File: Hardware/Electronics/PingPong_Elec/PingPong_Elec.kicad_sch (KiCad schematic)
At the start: 16 parts, among them M1 JGA25-371 12V, M2 JGA25-371 12V, M3 JGA25-371 12V, M4 MG996R, M5 MG996R, M6 MG996R, U1 DRV8871, U2 PCA9685PW, U5 DRV8871, U6 STM32F103RBTx LQFP64, U7 DRV8871

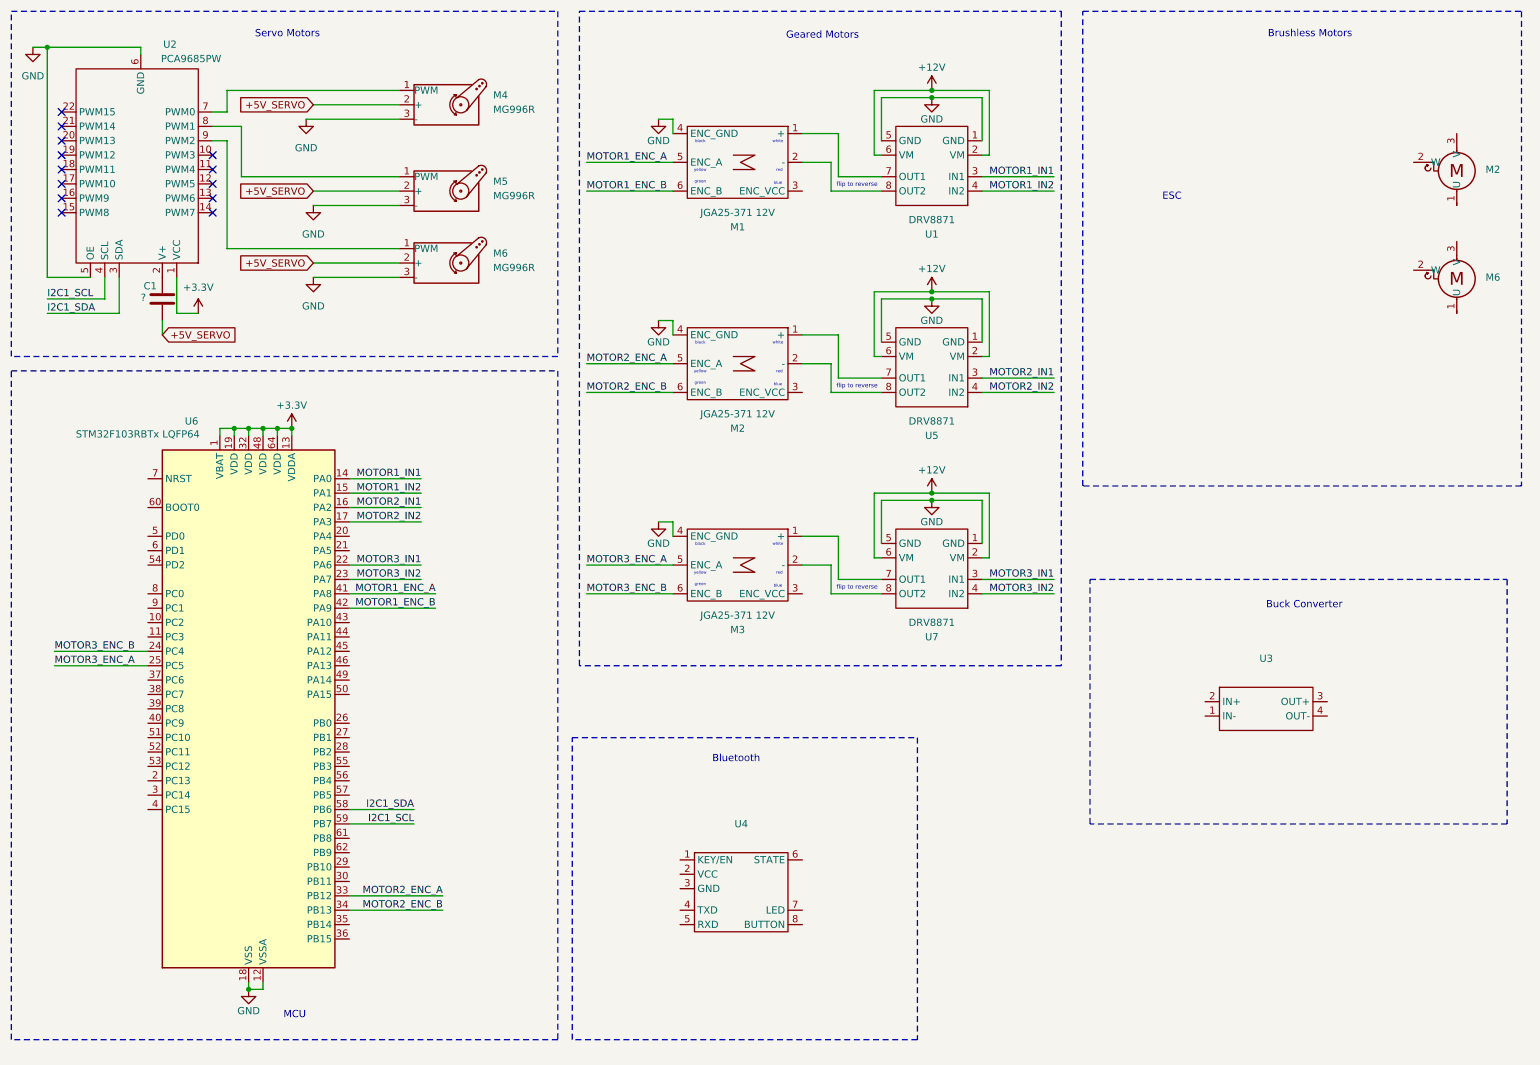
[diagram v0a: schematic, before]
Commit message: wired all schematic diagrams, adding bypass and decoupling caps
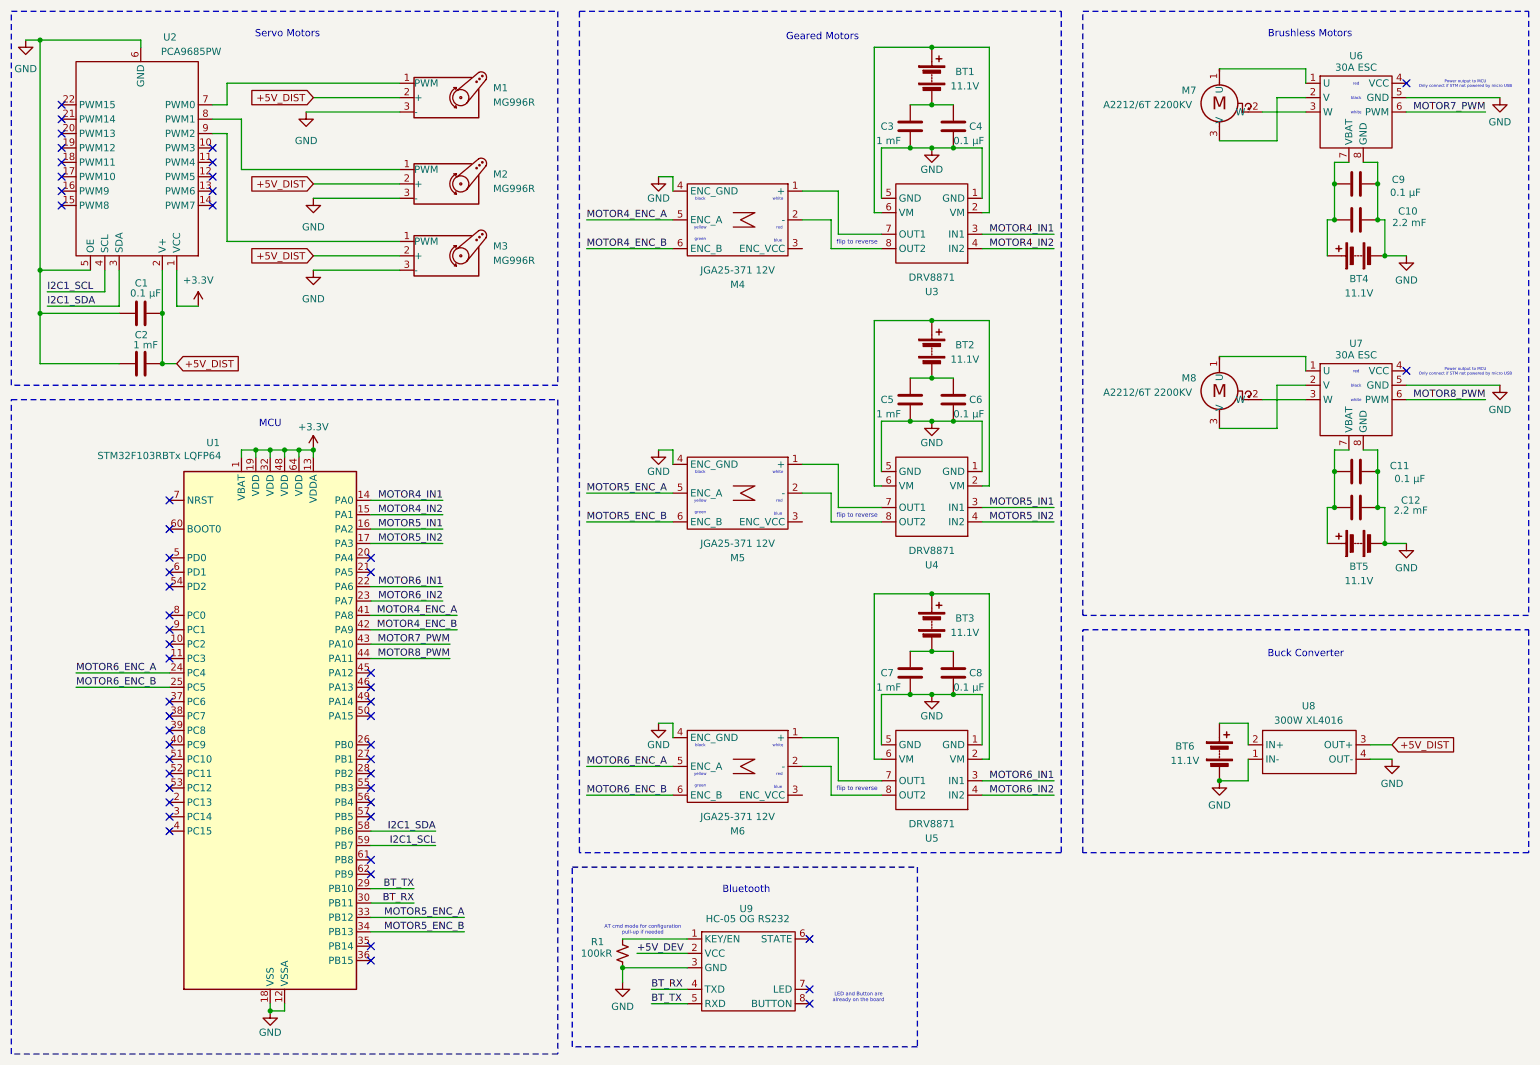
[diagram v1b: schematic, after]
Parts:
- removed M6: ~, symbol Motors:Motor_BLDC_3Phase
- added BT1, BT2, BT3, BT4, BT5, BT6: 11.1V, symbol Device:Battery
- added C1, C11, C4, C6, C8, C9: 0.1 µF, symbol Device:C
- added C10, C12: 2.2 mF, symbol Device:C
- added C3, C5, C7: 1 mF, symbol Device:C
- added M8: A2212/6T 2200KV, symbol Motors:Motor_BLDC_3Phase
- added R1: 100kR, symbol Device:R_Small_US
- added U6, U7: 30A ESC, symbol Motors:3Phase_ESC
- C2: renamed from C1; value ? -> 1 mF
- M7: renamed from M2; value ~ -> A2212/6T 2200KV
- U8: renamed from U3; value ~ -> 300W XL4016
- U9: renamed from U4; value ~ -> HC-05 OG RS232
- renumbered M4 to M1, M5 to M2, M6 to M3, M1 to M4, M2 to M5, M3 to M6, U6 to U1, U1 to U3, U5 to U4, U7 to U5
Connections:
- net +5V_SERVO is gone; now on net +5V_DIST: C2.2, M1.2 (+), M2.2 (+), M3.2 (+)
- net GND: now also C2.1, U8.1 (IN-), U8.4 (OUT-), U9.3 (GND), BT4.2 (-), BT5.2 (-), BT6.2 (-), C1.1, C10.2, C11.1, C12.2, C3.1, C4.1, C5.1, C6.1, C7.1, C8.1, C9.1, R1.2, U6.5 (GND), U6.8 (GND), U7.5 (GND), U7.8 (GND)
- net at U9.1 (KEY/EN): now also R1.1
- net +5V_DEV: now reaches U9.2 (VCC)
- net BT_RX: now reaches U9.4 (TXD)
- net BT_RX: now also U1.30 (PB11)
- net BT_TX: now reaches U9.5 (RXD)
- net BT_TX: now also U1.29 (PB10)
- net +5V_DIST: now reaches U2.2 (V+)
- net +5V_DIST: now also U8.3 (OUT+), C1.2; no longer C2.1
- net at U8.2 (IN+): now also BT6.1 (+)
- net at M7.1 (U): now also U6.1 (U)
- net at M7.2 (W): now also U6.3 (W)
- net at M7.3 (V): now also U6.2 (V)
- net MOTOR7_PWM: now reaches U1.43 (PA10)
- net MOTOR7_PWM: now also U6.6 (PWM)
- net MOTOR8_PWM: now reaches U1.44 (PA11)
- net MOTOR8_PWM: now also U7.6 (PWM)
- removed net +12V: U3.2 (VM), U3.6 (VM), U4.2 (VM), U4.6 (VM), U5.2 (VM), U5.6 (VM)
- net MOTOR1_ENC_A renamed MOTOR4_ENC_A
- net MOTOR1_ENC_B renamed MOTOR4_ENC_B
- net MOTOR1_IN1 renamed MOTOR4_IN1
- net MOTOR1_IN2 renamed MOTOR4_IN2
- net MOTOR2_ENC_A renamed MOTOR5_ENC_A
- net MOTOR2_ENC_B renamed MOTOR5_ENC_B
- net MOTOR2_IN1 renamed MOTOR5_IN1
- net MOTOR2_IN2 renamed MOTOR5_IN2
- net MOTOR3_ENC_A renamed MOTOR6_ENC_A
- net MOTOR6_ENC_A: now also U1.24 (PC4); no longer U1.25 (PC5)
- net MOTOR3_ENC_B renamed MOTOR6_ENC_B
- net MOTOR6_ENC_B: now also U1.25 (PC5); no longer U1.24 (PC4)
- net MOTOR3_IN1 renamed MOTOR6_IN1
- net MOTOR3_IN2 renamed MOTOR6_IN2
- new net: BT2.1 (+), U4.2 (VM), U4.6 (VM)
- new net: BT3.2 (-), C7.2, C8.2
- new net: BT5.1 (+), C11.2, C12.1, U7.7 (VBAT)
- new net: BT2.2 (-), C5.2, C6.2
- new net: BT1.1 (+), U3.2 (VM), U3.6 (VM)
- new net: BT1.2 (-), C3.2, C4.2
- new net: BT3.1 (+), U5.2 (VM), U5.6 (VM)
- new net: M8.1 (U), U7.1 (U)
- new net: M8.2 (W), U7.3 (W)
- new net: M8.3 (V), U7.2 (V)
- new net: BT4.1 (+), C10.1, C9.2, U6.7 (VBAT)
- no-connect marks 13 -> 53
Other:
- note added: "AT cmd mode for configuration pull-up if needed"
- note added: "LED and Button are already on the board"
- note added: "Power output to MCU Only connect if STM not powered by micro USB"
- note removed: "ESC"
- moved on the sheet: C2, M1, M2, M3, M4, M5, M6, M7, U1, U2, U3, U4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
